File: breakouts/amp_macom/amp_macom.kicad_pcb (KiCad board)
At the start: 4 copper layers, 18.5 x 18.5 mm, 8 parts, among them P1 CONN_01X02, U1 CONN_SMA, U2 CMM0511-QT-0G0T, U3 CONN_SMA

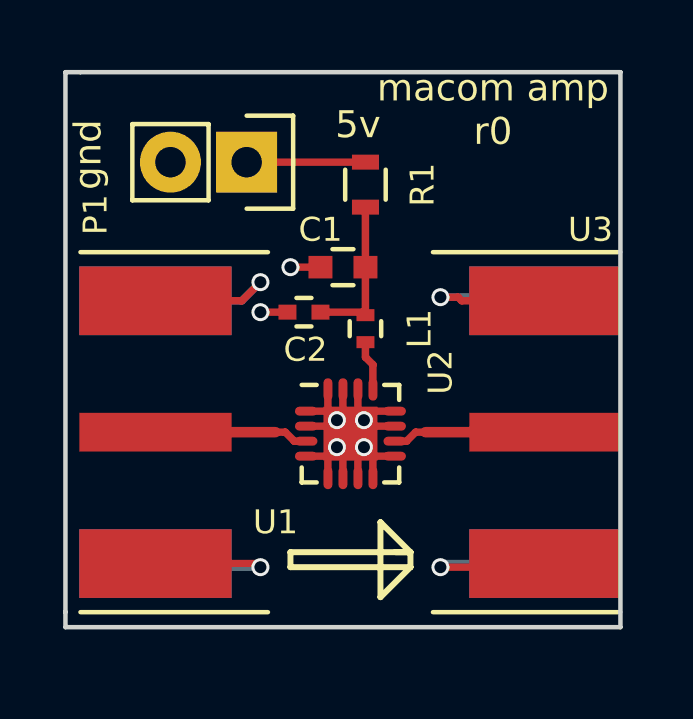
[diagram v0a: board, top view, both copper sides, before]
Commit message: work on ad9864 schematic, vco and if
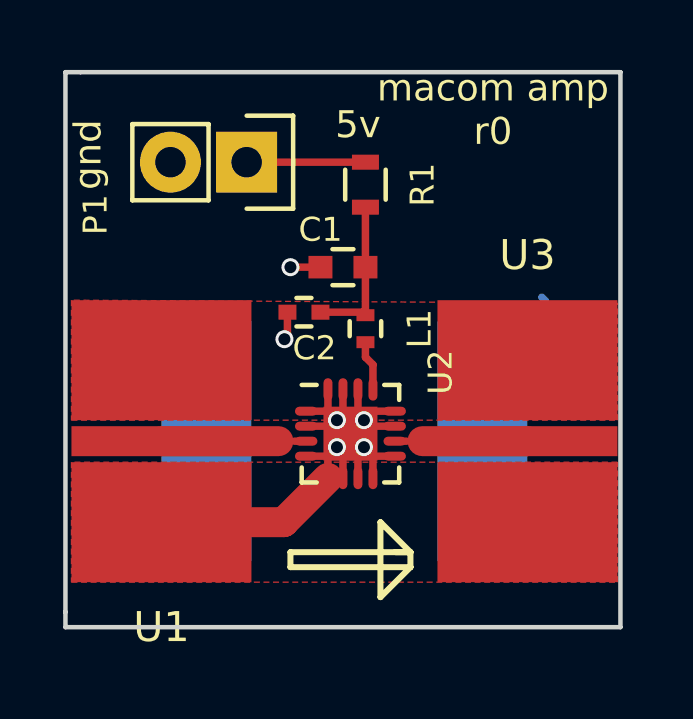
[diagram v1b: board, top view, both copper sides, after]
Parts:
- U1, U3: footprint vna_footprints:732511150_sma_thin -> vna_footprints:SMA_CPW_1MM_.2MM
- moved U3 0.67 mm to (146.9, 105.3)
- moved U1 0.36 mm to (134.7, 105.3)
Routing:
- net GND: track 44.1 -> 21.7 mm, vias 10 -> 6
- net Net-(U2-Pad10): track 5.15 -> 3.89 mm
- net Net-(U1-Pad1): track 5.15 -> 4.29 mm
- added copper zone on F.Cu, net GND
- added copper zone on In2.Cu, net GND
- removed copper zone on In1.Cu, net GND
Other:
- rule trace_min: 0.2 -> 0.15
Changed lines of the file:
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@@
 (kicad_pcb (version 4) (host pcbnew 4.0.2-stable)
   (general
-    (links 34)
-    (no_connects 17)
-    (area 131.2825 91.858333 150.275001 112.835)
+    (links 32)
+    (no_connects 2)
+    (area 131.424999 92.924999 150.075001 111.575001)
     (thickness 1.6)
     (drawings 17)
-    (tracks 68)
+    (tracks 49)
     (zones 0)
     (modules 8)
@@
     (last_trace_width 0.25)
     (user_trace_width 0.35)
+    (user_trace_width 1)
     (trace_clearance 0.2)
-    (zone_clearance 0.508)
+    (zone_clearance 0.2)
     (zone_45_only no)
-    (trace_min 0.2)
+    (trace_min 0.15)
     (segment_width 0.2)
     (edge_width 0.15)
@@
     (tags "capacitor 0402")
     (attr smd)
-    (fp_text reference C2 (at -0.05 -1.25 180) (layer F.SilkS)
+    (fp_text reference C2 (at -0.35 -1.2 180) (layer F.SilkS)
       (effects (font (size 0.8 0.8) (thickness 0.15)))
     )
@@
     )
   )
-  (module vna_footprints:732511150_sma_thin (layer F.Cu)
-    (at 134.5 105 270)
-    (fp_text reference U1 (at 3 -4 360) (layer F.SilkS)
-      (effects (font (size 0.8 0.8) (thickness 0.15)))
-    )
-    (fp_text value CONN_SMA (at 7 -3.5 360) (layer F.Fab)
-      (effects (font (size 0.8 0.8) (thickness 0.15)))
-    )
-    (fp_line (start 6 2.5) (end 6 -3.75) (layer F.SilkS) (width 0.15))
-    (fp_line (start -6 2.5) (end -6 -3.75) (layer F.SilkS) (width 0.15))
-    (pad 1 smd rect (at 0 0 270) (size 1.29 5.08) (layers F.Cu F.Paste F.Mask)
-      (net 5 "Net-(U1-Pad1)"))
-    (pad 2 smd rect (at 4.38 0 270) (size 2.29 5.08) (layers F.Cu F.Paste F.Mask)
-      (net 2 GND))
-    (pad 3 smd rect (at -4.38 0 270) (size 2.29 5.08) (layers F.Cu F.Paste F.Mask)
-      (net 2 GND))
-    (pad 4 smd rect (at -4.38 0 270) (size 2.29 5.08) (layers B.Cu B.Paste B.Mask)
-      (net 2 GND))
-    (pad 5 smd rect (at 4.38 0 270) (size 2.29 5.08) (layers B.Cu B.Paste B.Mask)
-      (net 2 GND))
-  )
   (module Housings_DFN_QFN:QFN-16-1EP_3x3mm_Pitch0.5mm (layer F.Cu)
     (at 141 105.05)
@@
     )
   )
-  (module vna_footprints:732511150_sma_thin (layer F.Cu)
-    (at 147.5 105 90)
-    (fp_text reference U3 (at 6.75 1.5 180) (layer F.SilkS)
-      (effects (font (size 0.8 0.8) (thickness 0.15)))
-    )
-    (fp_text value CONN_SMA (at 7 -3.5 180) (layer F.Fab)
-      (effects (font (size 0.8 0.8) (thickness 0.15)))
-    )
-    (fp_line (start 6 2.5) (end 6 -3.75) (layer F.SilkS) (width 0.15))
-    (fp_line (start -6 2.5) (end -6 -3.75) (layer F.SilkS) (width 0.15))
-    (pad 1 smd rect (at 0 0 90) (size 1.29 5.08) (layers F.Cu F.Paste F.Mask)
+  (module vna_footprints:SMA_CPW_1MM_.2MM (layer F.Cu)
+    (at 134.7 105.3 270)
+    (fp_text reference U1 (at 6.2 0 360) (layer F.SilkS)
+      (effects (font (size 1 1) (thickness 0.15)))
+    )
+    (fp_text value CONN_SMA (at -6.5 4.6 360) (layer F.Fab)
+      (effects (font (size 1 1) (thickness 0.15)))
+    )
+    (pad 1 smd rect (at 0 0 270) (size 1 6) (layers F.Cu F.Paste F.Mask)
+      (net 5 "Net-(U1-Pad1)"))
+    (pad 2 smd rect (at -2.7 0 270) (size 4 6) (layers F.Cu F.Paste F.Mask)
+      (net 2 GND))
+    (pad 2 smd rect (at 2.7 0 270) (size 4 6) (layers F.Cu F.Paste F.Mask)
+      (net 2 GND))
+    (pad 3 smd rect (at 0 -1.5 180) (size 3 8) (layers B.Cu B.Paste B.Mask)
+      (net 2 GND))
+  )
+  (module vna_footprints:SMA_CPW_1MM_.2MM (layer F.Cu)
+    (at 146.9 105.3 90)
+    (fp_text reference U3 (at 6.2 0 180) (layer F.SilkS)
+      (effects (font (size 1 1) (thickness 0.15)))
+    )
+    (fp_text value CONN_SMA (at -6.5 4.6 180) (layer F.Fab)
+      (effects (font (size 1 1) (thickness 0.15)))
+    )
+    (pad 1 smd rect (at 0 0 90) (size 1 6) (layers F.Cu F.Paste F.Mask)
       (net 6 "Net-(U2-Pad10)"))
-    (pad 2 smd rect (at 4.38 0 90) (size 2.29 5.08) (layers F.Cu F.Paste F.Mask)
-      (net 2 GND))
-    (pad 3 smd rect (at -4.38 0 90) (size 2.29 5.08) (layers F.Cu F.Paste F.Mask)
-      (net 2 GND))
-    (pad 4 smd rect (at -4.38 0 90) (size 2.29 5.08) (layers B.Cu B.Paste B.Mask)
-      (net 2 GND))
-    (pad 5 smd rect (at 4.38 0 90) (size 2.29 5.08) (layers B.Cu B.Paste B.Mask)
+    (pad 2 smd rect (at -2.7 0 90) (size 4 6) (layers F.Cu F.Paste F.Mask)
+      (net 2 GND))
+    (pad 2 smd rect (at 2.7 0 90) (size 4 6) (layers F.Cu F.Paste F.Mask)
+      (net 2 GND))
+    (pad 3 smd rect (at 0 -1.5) (size 3 8) (layers B.Cu B.Paste B.Mask)
       (net 2 GND))
   )
@@
   (gr_line (start 131.5 111.5) (end 150 111.5) (layer Edge.Cuts) (width 0.15))
   (gr_line (start 131.5 111) (end 131.5 111.5) (layer Edge.Cuts) (width 0.15))
+  (segment (start 147.38 100.5) (end 147.5 100.62) (width 0.25) (layer B.Cu) (net 0))
+  (segment (start 134.62 109.5) (end 134.5 109.38) (width 0.25) (layer B.Cu) (net 0))
   (segment (start 140 101) (end 141.4 101) (width 0.25) (layer F.Cu) (net 1))
   (segment (start 141.4 101) (end 141.5 101.1) (width 0.25) (layer F.Cu) (net 1))
   (segment (start 141.5 101.1) (end 141.5 99.5) (width 0.25) (layer F.Cu) (net 1))
   (segment (start 141.5 97.5) (end 141.5 99.5) (width 0.25) (layer F.Cu) (net 1))
+  (segment (start 134.7 108) (end 138.775 108) (width 1) (layer F.Cu) (net 2))
+  (segment (start 138.775 108) (end 140.25 106.525) (width 1) (layer F.Cu) (net 2))
+  (segment (start 138.9 101.8) (end 138.8 101.9) (width 0.25) (layer F.Cu) (net 2))
+  (via (at 138.8 101.9) (size 0.6) (drill 0.4) (layers F.Cu B.Cu) (net 2))
+  (segment (start 138.9 101) (end 138.9 101.8) (width 0.25) (layer F.Cu) (net 2))
   (via (at 140.55 105.5) (size 0.6) (drill 0.4) (layers F.Cu B.Cu) (net 2))
   (via (at 141.45 105.5) (size 0.6) (drill 0.4) (layers F.Cu B.Cu) (net 2))
@@
   (segment (start 140.25 104.3) (end 140.55 104.6) (width 0.25) (layer F.Cu) (net 2))
   (segment (start 140.25 103.575) (end 140.25 104.3) (width 0.25) (layer F.Cu) (net 2))
-  (segment (start 144 100.5) (end 147.38 100.5) (width 0.25) (layer B.Cu) (net 2))
-  (segment (start 147.38 100.5) (end 147.5 100.62) (width 0.25) (layer B.Cu) (net 2))
-  (segment (start 144.59 100.5) (end 144 100.5) (width 0.25) (layer F.Cu) (net 2))
-  (via (at 144 100.5) (size 0.6) (drill 0.4) (layers F.Cu B.Cu) (net 2))
-  (segment (start 147.5 100.62) (end 144.71 100.62) (width 0.25) (layer F.Cu) (net 2))
-  (segment (start 144.71 100.62) (end 144.59 100.5) (width 0.25) (layer F.Cu) (net 2))
-  (segment (start 144 109.5) (end 147.38 109.5) (width 0.25) (layer F.Cu) (net 2))
   (segment (start 147.38 109.5) (end 147.5 109.38) (width 0.25) (layer F.Cu) (net 2))
-  (segment (start 147.5 109.38) (end 144.12 109.38) (width 0.25) (layer B.Cu) (net 2))
-  (segment (start 144.12 109.38) (end 144 109.5) (width 0.25) (layer B.Cu) (net 2))
-  (via (at 144 109.5) (size 0.6) (drill 0.4) (layers F.Cu B.Cu) (net 2))
-  (segment (start 138 109.5) (end 134.62 109.5) (width 0.25) (layer B.Cu) (net 2))
-  (segment (start 134.62 109.5) (end 134.5 109.38) (width 0.25) (layer B.Cu) (net 2))
-  (segment (start 134.5 109.38) (end 137.88 109.38) (width 0.25) (layer F.Cu) (net 2))
-  (segment (start 137.88 109.38) (end 138 109.5) (width 0.25) (layer F.Cu) (net 2))
-  (via (at 138 109.5) (size 0.6) (drill 0.4) (layers F.Cu B.Cu) (net 2))
-  (segment (start 134.5 100.62) (end 137.38 100.62) (width 0.25) (layer F.Cu) (net 2))
-  (segment (start 137.38 100.62) (end 138 100) (width 0.25) (layer F.Cu) (net 2))
-  (segment (start 134.5 100.62) (end 137.38 100.62) (width 0.25) (layer B.Cu) (net 2))
-  (segment (start 137.38 100.62) (end 138 100) (width 0.25) (layer B.Cu) (net 2))
-  (via (at 138 100) (size 0.6) (drill 0.4) (layers F.Cu B.Cu) (net 2))
-  (segment (start 138.9 101) (end 138 101) (width 0.25) (layer F.Cu) (net 2))
-  (via (at 138 101) (size 0.6) (drill 0.4) (layers F.Cu B.Cu) (net 2))
   (via (at 139 99.5) (size 0.6) (drill 0.4) (layers F.Cu B.Cu) (net 2))
   (segment (start 140 99.5) (end 139 99.5) (width 0.25) (layer F.Cu) (net 2))
@@
   (segment (start 141.75 103.575) (end 141.75 102.75) (width 0.25) (layer F.Cu) (net 3))
   (segment (start 137.54 96) (end 141.5 96) (width 0.25) (layer F.Cu) (net 4))
-  (segment (start 138.5 105) (end 134.5 105) (width 0.35) (layer F.Cu) (net 5))
-  (segment (start 138.828235 105) (end 138.5 105) (width 0.25) (layer F.Cu) (net 5))
+  (segment (start 134.7 105.3) (end 138.597905 105.3) (width 1) (layer F.Cu) (net 5))
   (segment (start 139.525 105.3) (end 139.128235 105.3) (width 0.25) (layer F.Cu) (net 5))
-  (segment (start 139.128235 105.3) (end 138.828235 105) (width 0.25) (layer F.Cu) (net 5))
-  (segment (start 143.5 105) (end 147.5 105) (width 0.35) (layer F.Cu) (net 6))
-  (segment (start 143.171765 105) (end 143.5 105) (width 0.25) (layer F.Cu) (net 6))
+  (segment (start 146.9 105.3) (end 143.402095 105.3) (width 1) (layer F.Cu) (net 6))
   (segment (start 142.475 105.3) (end 142.871765 105.3) (width 0.25) (layer F.Cu) (net 6))
-  (segment (start 142.871765 105.3) (end 143.171765 105) (width 0.25) (layer F.Cu) (net 6))
-  (zone (net 2) (net_name GND) (layer In1.Cu) (hatch edge 0.508)
+  (zone (net 2) (net_name GND) (layer In2.Cu) (hatch edge 0.508)
     (connect_pads yes (clearance 0.508))
     (min_thickness 0.254)
@@
       )
     )
+  )
+  (zone (net 2) (net_name GND) (layer F.Cu) (hatch edge 0.508)
+    (connect_pads yes (clearance 0.2))
+    (min_thickness 0.254)
+    (fill yes (arc_segments 16) (thermal_gap 0.508) (thermal_bridge_width 0.508))
+    (polygon
+      (pts
+        (xy 131.7 104.6) (xy 149.9 104.6) (xy 149.9 100.7) (xy 131.7 100.6)
+      )
+    )
+  )
+  (zone (net 2) (net_name GND) (layer F.Cu) (hatch edge 0.508)
+    (connect_pads yes (clearance 0.2))
+    (min_thickness 0.254)
+    (fill yes (arc_segments 16) (thermal_gap 0.508) (thermal_bridge_width 0.508))
+    (polygon
+      (pts
+        (xy 131.7 106) (xy 131.7 110) (xy 149.9 110) (xy 149.9 106) (xy 141.6 106)
+        (xy 141.6 106)
+      )
+    )
